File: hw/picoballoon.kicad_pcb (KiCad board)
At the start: 2 copper layers, 51.2 x 20 mm, 30 parts, among them J0 PinSocket_1x01_P2.00mm_Vertic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, J1 Conn_ARM_JTAG_SWD_10, J2 Conn_01x01, J3 Conn_01x01, J4 u.fl, U1 YFF0006AFAD, U2 K32L2B21VLH0A, U3 L96-M33, U4 INNOCOMM-SN10-11, U5 MS561101BA03-50

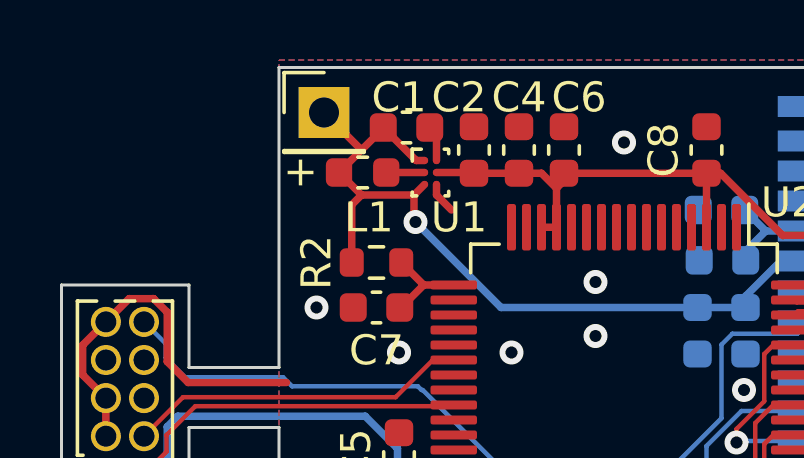
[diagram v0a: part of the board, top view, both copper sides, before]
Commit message: part #s
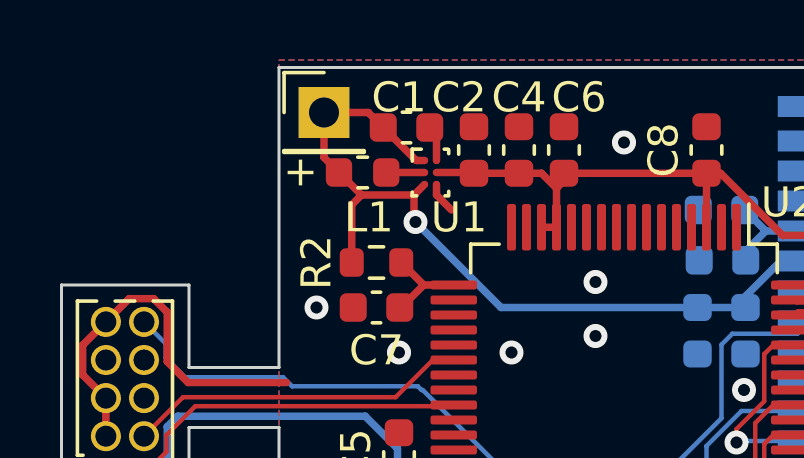
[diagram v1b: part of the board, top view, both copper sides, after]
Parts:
- U1: value YFF0006AFAD -> TPS610994YFFR
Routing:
- net +BATT: track 27.5 -> 28.0 mm

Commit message: exports
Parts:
- J0: value PinSocket_1x01_P2.00mm_Vertical -> (none)
- J2, J3: value Conn_01x01 -> ~
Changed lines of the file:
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@@
         (effects (font (size 1 1) (thickness 0.15)))
     )
-    (fp_text value "Conn_01x01" (at 0 2.33) (layer "F.Fab")
+    (fp_text value "~" (at 0 2.33) (layer "F.Fab")
         (effects (font (size 1 1) (thickness 0.15)))
     )
@@
     (descr "Through hole straight socket strip, 1x01, 2.00mm pitch, single row (from Kicad 4.0.7), script generated")
     (tags "Through hole socket strip THT 1x01 2.00mm single row")
-    (attr through_hole)
+    (attr through_hole board_only exclude_from_bom)
     (fp_text reference "J0" (at 0 -2.5) (layer "F.SilkS") hide
         (effects (font (size 1 1) (thickness 0.15)))
     )
-    (fp_text value "PinSocket_1x01_P2.00mm_Vertical" (at 0 2.5) (layer "F.Fab")
+    (fp_text value "" (at 0 2.5) (layer "F.Fab")
         (effects (font (size 1 1) (thickness 0.15)))
     )
@@
         (effects (font (size 1 1) (thickness 0.15)))
     )
-    (fp_text value "Conn_01x01" (at 0 2.33) (layer "F.Fab")
-        (effects (font (size 1 1) (thickness 0.15)))
-    )
+    (fp_text value "~" (at 0 2.33) (layer "F.Fab")
+        (effects (font (size 1 1) (thickness 0.15)))
+    )
